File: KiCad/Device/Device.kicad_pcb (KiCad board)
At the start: 2 copper layers, 109.6 x 72.2 mm, 27 parts, among them IC1 ATTINY167-XUR, J1 Mikrofon, J2 Lysføler, J3 Optisk sensor, J4 Fugtføler, J5 VCC, J6 ESP8266(wifi), SW1 SW_MEC_5E, SW3 SW_MEC_5E, SW4 SW_DIP_x02, Y1 Crystal

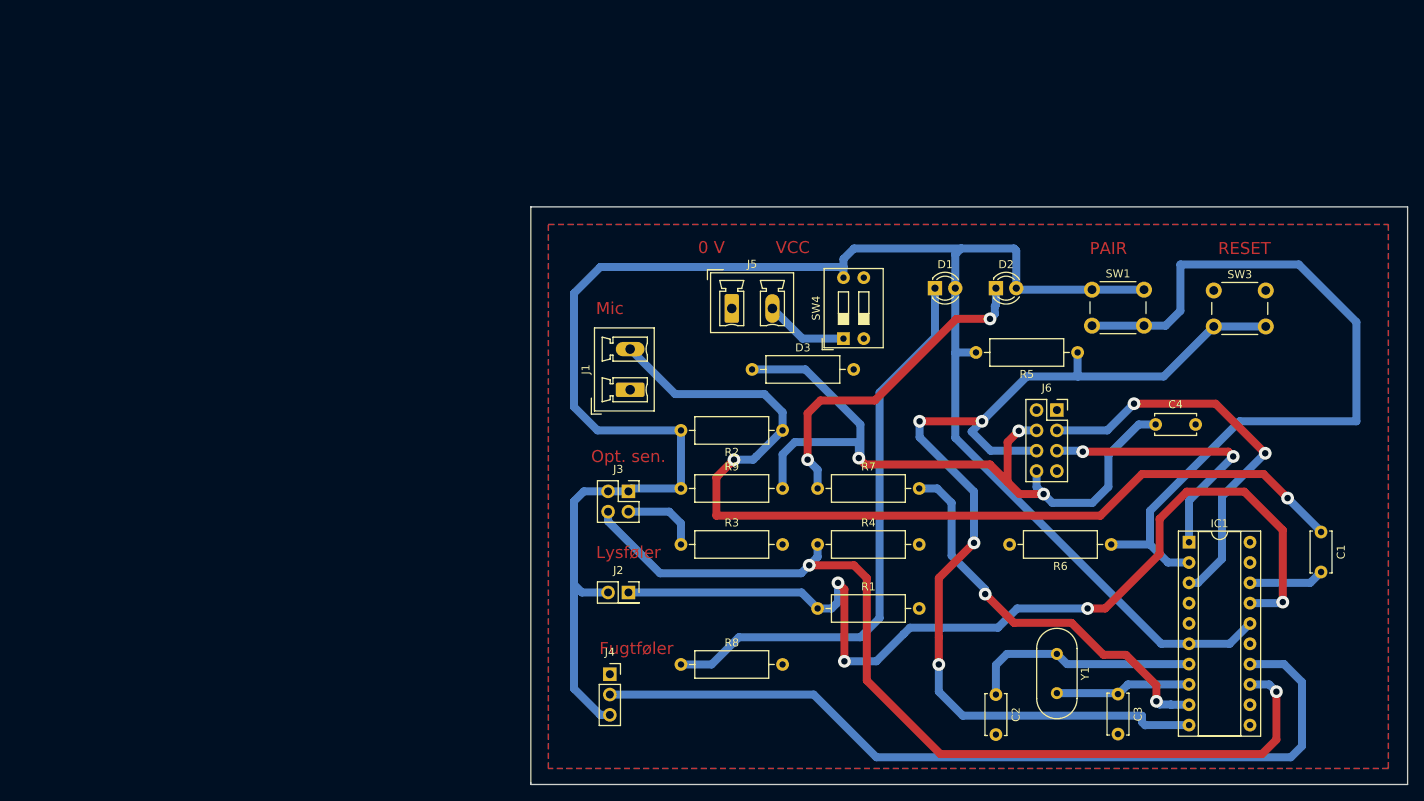
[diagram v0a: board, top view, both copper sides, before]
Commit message: save
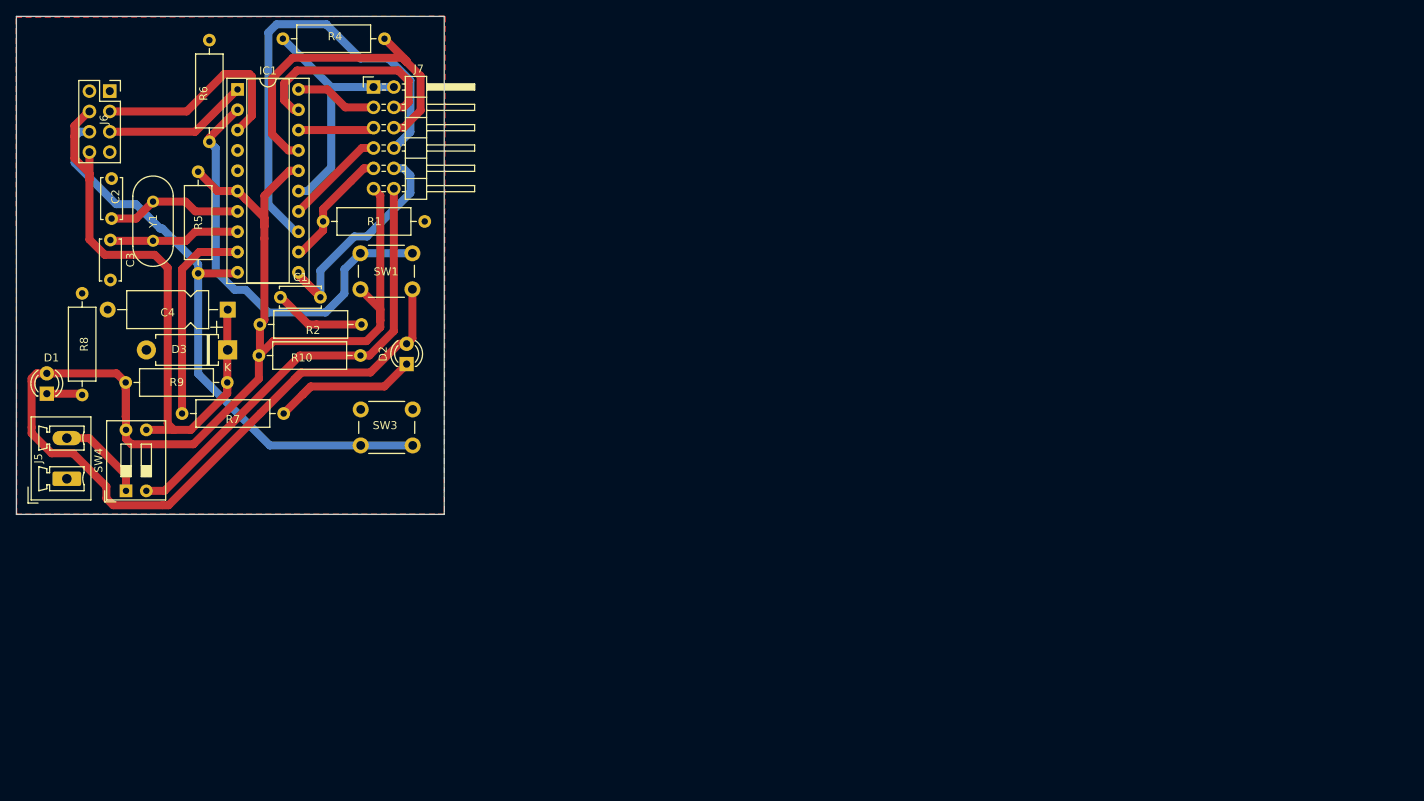
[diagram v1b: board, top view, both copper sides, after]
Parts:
- removed J1: Mikrofon, Connector_Phoenix_MC_HighVoltage:PhoenixContact_MCV_1,5_2-G-5.08_1x02_P5.08mm_Vertical
- removed J2: Lysføler, Connector_PinSocket_2.54mm:PinSocket_2x01_P2.54mm_Vertical
- removed J3: Optisk sensor, Connector_PinSocket_2.54mm:PinSocket_2x02_P2.54mm_Vertical
- removed J4: Fugtføler, Connector_PinSocket_2.54mm:PinSocket_1x03_P2.54mm_Vertical
- removed R3: 10k, Resistor_THT:R_Axial_DIN0309_L9.0mm_D3.2mm_P12.70mm_Horizontal
- added J7: Conn_02x06_Counter_Clockwise, Connector_PinHeader_2.54mm:PinHeader_2x06_P2.54mm_Horizontal, F.Cu at (77.1, 35.8)
- added R10: 15, Resistor_THT:R_Axial_DIN0309_L9.0mm_D3.2mm_P12.70mm_Horizontal, F.Cu at (62.8, 69.4)
- C4: footprint Capacitor_THT:C_Disc_D5.0mm_W2.5mm_P5.00mm -> Capacitor_THT:CP_Axial_L10.0mm_D4.5mm_P15.00mm_Horizontal
- D3: footprint Resistor_THT:R_Axial_DIN0309_L9.0mm_D3.2mm_P12.70mm_Horizontal -> Diode_THT:D_DO-15_P10.16mm_Horizontal
- moved C3 138.1 mm to (44.2, 54.9)
- moved C1 133.3 mm to (65.5, 62.1), turned to 0 degrees
- moved IC1 131.7 mm to (60.1, 36.1)
- moved Y1 126.3 mm to (49.6, 50.1)
- moved C2 125.5 mm to (44.4, 52.3), turned to 90 degrees
- moved J6 124.9 mm to (44.2, 36.3)
- moved R6 123.5 mm to (56.6, 42.7), turned to 90 degrees
- moved C4 116.9 mm to (58.9, 63.6), turned to 180 degrees
- moved D1 111.8 mm to (36.3, 74.2), turned to 90 degrees
- moved R5 110.4 mm to (55.2, 59.1), turned to 90 degrees
- moved SW3 107.7 mm to (75.5, 76.1)
- moved SW4 91.7 mm to (46.2, 86.3)
- moved J5 85.8 mm to (38.8, 84.8), turned to 90 degrees
- moved SW1 85.0 mm to (82.0, 61.1), turned to 180 degrees
- moved R4 83.2 mm to (78.5, 29.8), turned to 180 degrees
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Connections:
- net GrønLED renamed LED_G
- net Net-(C1-Pad1) renamed MIC
- C1 pad 2: Mic_out -> UP7
- C4 pad 1: +3,3V -> +3V3
- D3 pad 1: +3,3V -> +3V3
- IC1 pad 11: unconnected-(IC1-Pad11) -> UP7
- IC1 pad 12: unconnected-(IC1-Pad12) -> PHOTRAN
- IC1 pad 13: Op.Sensor_out -> UP5
- IC1 pad 14: Fugt_out -> UP4
- IC1 pad 17: Photo_out -> OPTISK
- IC1 pad 18: Mic_out -> UP2
- IC1 pad 19: unconnected-(IC1-Pad19) -> UP1
- IC1 pad 20: unconnected-(IC1-Pad20) -> DHT11
- J6 pad 4: +3,3V -> +3V3
- J6 pad 8: +3,3V -> +3V3
- R1 pad 1: Photo_out -> PHOTRAN
- R4 pad 1: Op.Sensor_out -> OPTISK
- R9 pad 1: +5V -> +3V3
- R9 pad 2: +3,3V -> +5V
- SW4 pad 2: unconnected-(SW4-Pad2) -> UPWR
- SW4 pad 3: unconnected-(SW4-Pad3) -> +3V3
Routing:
- net Photo_out: track 121.2 -> 0.00 mm, vias 4 -> 0
- net Op.Sensor_out: track 118.6 -> 0.00 mm, vias 2 -> 0
- net MIC: track 120.9 -> 11.6 mm, vias 2 -> 0
- net Fugt_out: track 105.8 -> 0.00 mm
- net +3,3V: track 95.5 -> 0.00 mm, vias 3 -> 0
- net +3V3: track 0.00 -> 75.4 mm
- net Net-(D1-Pad1): track 71.3 -> 4.49 mm
- net Reset: track 134.1 -> 75.2 mm, vias 4 -> 0
- net UP5: track 0.00 -> 57.1 mm
- net UPWR: track 0.00 -> 57.0 mm
- net Button01: track 100.3 -> 53.5 mm
- net OPTISK: track 0.00 -> 45.0 mm
- net +5V: track 239.5 -> 200.4 mm
- net GND: track 0.00 -> 31.7 mm
- net UP7: track 0.00 -> 31.6 mm
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- removed copper zone on B.Cu, net GND
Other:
- board size 109.6 x 72.2 mm -> 53.5 x 62.2 mm
- board text removed: "0 V"
- board text removed: "Fugtføler"
- board text removed: "Lysføler"
- board text removed: "Mic"
- board text removed: "Opt. sen."
- board text removed: "PAIR"
- board text removed: "RESET"
- board text removed: "VCC"
